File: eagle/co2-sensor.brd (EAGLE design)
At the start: 34 x 30 mm, 14 parts, among them IC1 LM1117IMPX-3.3, J1 MH-Z19, U1 esp12e, U2 dht22

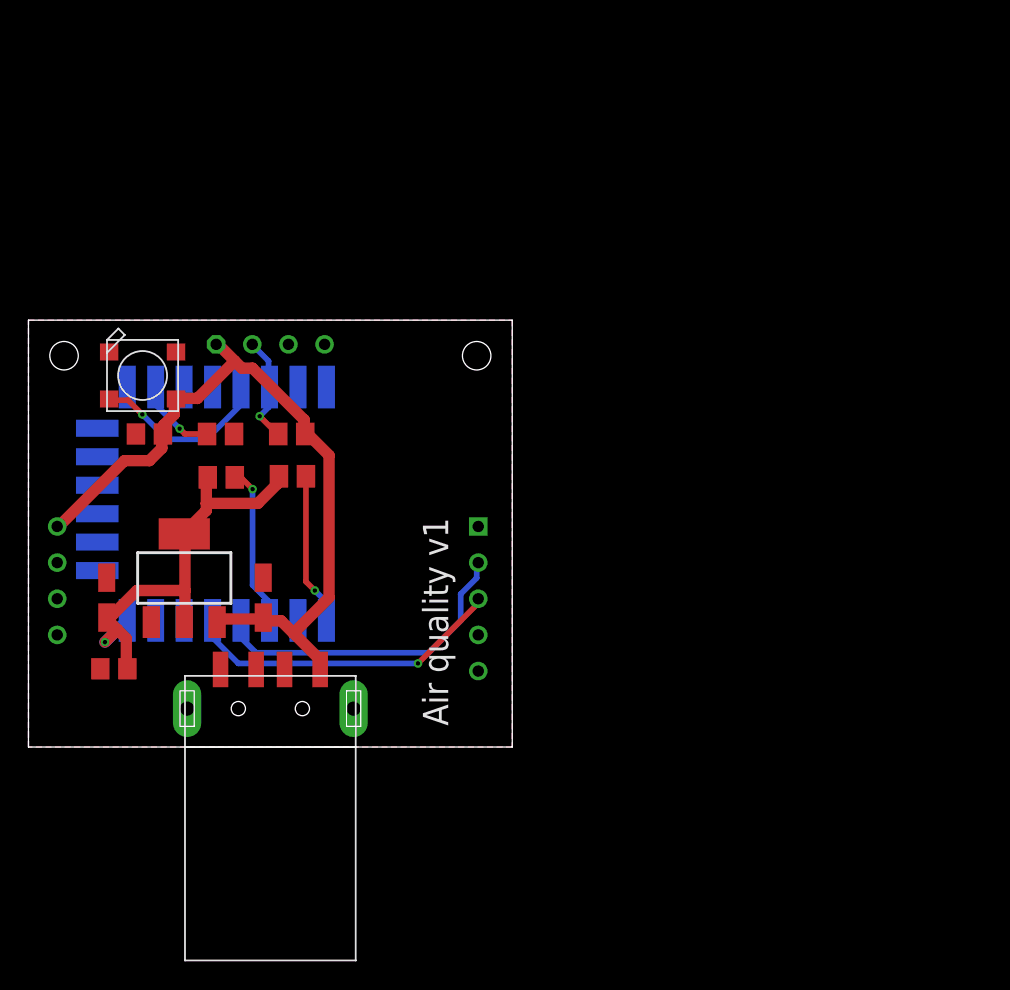
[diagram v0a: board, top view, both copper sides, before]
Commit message: .
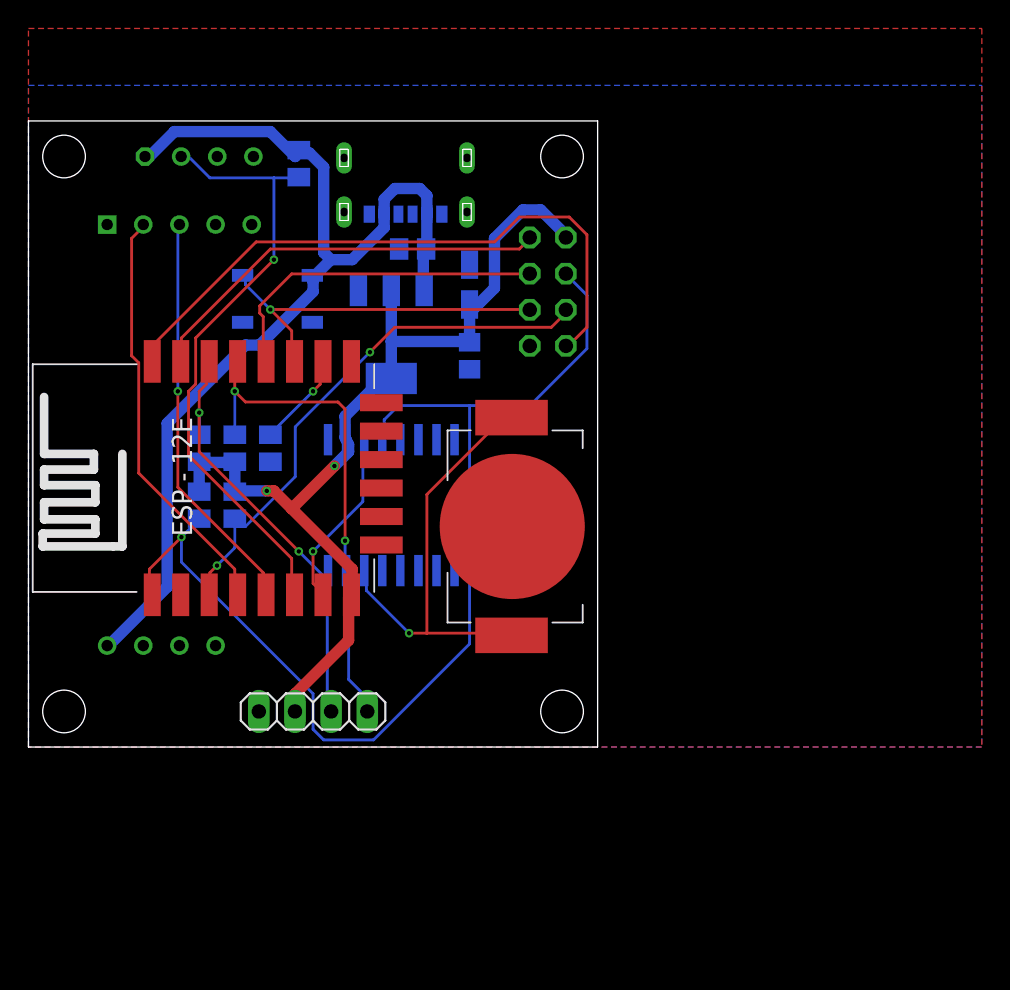
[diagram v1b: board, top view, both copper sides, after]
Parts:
- removed C1: 10mF, rcl:CT3216
- added BT1: BAT-HLD-012-SMT, BAT-HLD-012-SMT:BAT_BAT-HLD-012-SMT
- added IC2: (no value), DS3231_industrialberry:SOIC-16W
- added JP1: (no value), pinhead:1X04
- added JP2: (no value), pinhead:2X04
- added R5, R6: 4.7k, rcl:M0805
- C4: value 100n -> 10u
- LED1: value WS2812B_5050N -> WS2812B5050; device WS2812B:WS2812B-NARROW -> WS2812B:WS2812B
- U$1: value USB-A -> USB-C; device usb:USB-A-SMT -> USB-C:USB-C
- moved J1 50.0 mm to (19.5, 46.5), turned to 270 degrees
- moved U$1 45.0 mm to (26.5, 44.0), flipped to the bottom, turned to 180 degrees
- moved C2 33.7 mm to (31.0, 32.5), flipped to the bottom
- moved C3 33.3 mm to (31.0, 27.5), flipped to the bottom, turned to 270 degrees
- moved C4 22.6 mm to (27.0, 35.0), flipped to the bottom, turned to 0 degrees
- moved IC1 22.5 mm to (25.5, 29.0), flipped to the bottom, turned to 180 degrees
- moved R4 19.0 mm to (19.0, 41.0), flipped to the bottom, turned to 90 degrees
- moved U2 14.1 mm to (12.0, 41.5)
- moved LED1 10.9 mm to (17.5, 31.5), flipped to the bottom, turned to 180 degrees
- moved R1 4.53 mm to (14.5, 17.0), flipped to the bottom, turned to 270 degrees
- moved R3 3.64 mm to (17.0, 21.0), flipped to the bottom, turned to 270 degrees
- moved R2 2.49 mm to (12.0, 17.0), flipped to the bottom, turned to 270 degrees
- moved U1 1.91 mm to (14.5, 19.0), flipped to the top
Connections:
- removed net LED: LED1.4-DIN, U1.GPIO4
- removed net RESET: R1.2, U1.RESET
- new net CLOCK_INT: IC2.3, U1.GPIO13
- new net IO0: JP2.5, U1.GPIO0
- new net IO2: JP2.3, LED1.4-DIN, U1.GPIO2
- new net N$6: BT1.P1, BT1.P2, IC2.14
- new net RST: IC2.4, JP2.6, R2.2, U1.RESET
- new net RXD: JP2.7, U1.RXD0
- new net SCL: IC2.16, JP1.3, R6.2, U1.GPIO5
- new net SDA: IC2.15, JP1.4, R5.2, U1.GPIO4
- new net TXD: JP2.2, U1.TXD0
- net +3V3: now also IC2.2, JP1.2, JP2.8, R5.1, R6.1
- net +5V: now also U$1.A9, U$1.B9; no longer C1.+, U$1.P$6
- net CH_PD: now also JP2.4, R1.2; no longer R2.2
- net DHT22: now also U1.GPIO12; no longer U1.GPIO5
- net GND: now also BT1.N, IC2.10, IC2.11, IC2.12, IC2.13, IC2.5, IC2.6, IC2.7, IC2.8, IC2.9, JP1.1, JP2.1, U$1.A12, U$1.B12, U$1.P$10, U$1.P$7, U$1.P$8, U$1.P$9; no longer C1.-, U$1.P$1, U$1.P$2, U$1.P$3
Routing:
- net RST: track 0.00 -> 78.8 mm, vias 0 -> 1
- net TXD: track 0.00 -> 44.4 mm
- net +3V3: track 31.1 -> 68.7 mm, vias 1 -> 2
- net DHT22: track 7.64 -> 43.9 mm
- net SDA: track 0.00 -> 35.5 mm, vias 0 -> 2
- net SCL: track 0.00 -> 31.6 mm, vias 0 -> 2
- net N$6: track 0.00 -> 30.9 mm, vias 0 -> 1
- net RXD: track 0.00 -> 29.1 mm
- net CH_PD: track 11.3 -> 37.8 mm, vias 1 -> 2
- net IO2: track 0.00 -> 25.8 mm, vias 0 -> 1
- net IO0: track 0.00 -> 24.0 mm
- net +5V: track 53.4 -> 73.1 mm
- net CLOCK_INT: track 0.00 -> 12.7 mm, vias 0 -> 1
- net LED: track 12.7 -> 0.00 mm, vias 1 -> 0
- net RESET: track 10.7 -> 0.00 mm, vias 1 -> 0
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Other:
- board size 34 x 30 mm -> 40 x 44 mm
- board text removed: "Air quality v1"
